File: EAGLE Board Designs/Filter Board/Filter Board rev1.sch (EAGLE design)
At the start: 118 parts, among them J4 CONNECTOR-40__, J5 CONNECTOR-40__, U10 MAX7400, U11 MAX7400, U19 MAX7400, U20 MAX7400, U21 MAX7400, U22 MAX7400, U23 MAX7400, U24 MAX7400, U6 MAX7400, U7 MAX7400, U8 MAX7400, U9 MAX7400

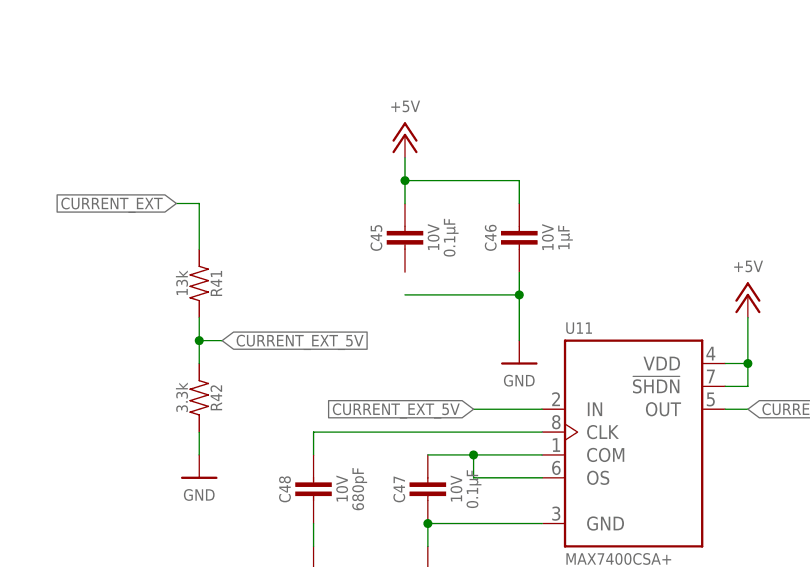
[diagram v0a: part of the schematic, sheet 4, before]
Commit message: quick fix
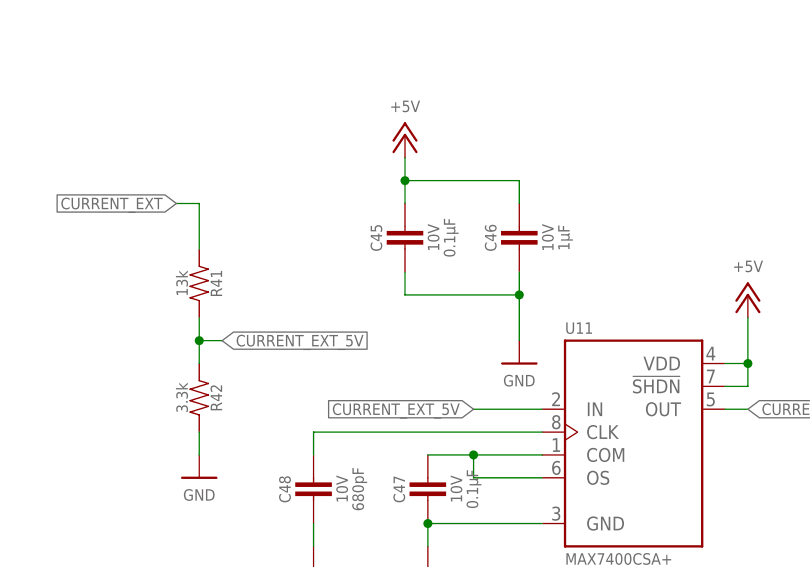
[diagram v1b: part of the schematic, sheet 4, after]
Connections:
- net GND: now also C45.2
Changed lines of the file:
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@@
 <pinref part="P139" gate="1" pin="GND"/>
 <pinref part="C46" gate="G$1" pin="2"/>
+<pinref part="C45" gate="G$1" pin="2"/>
+<wire x1="55.88" y1="53.34" x2="55.88" y2="50.8" width="0.1524" layer="91"/>
 </segment>
 <segment>

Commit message: inverted design
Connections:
- removed net GND1: R12.2, R16.2
- removed net GND2: R14.2, R18.2, R42.2, R44.2
- net GND: now also R12.2, R14.2, R16.2, R18.2, R44.2
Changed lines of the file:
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@@
 <pinref part="C10" gate="G$1" pin="2"/>
+</segment>
+<segment>
+<pinref part="P15" gate="1" pin="GND"/>
+<pinref part="R16" gate="G$1" pin="2"/>
+<wire x1="40.64" y1="73.66" x2="40.64" y2="76.2" width="0.1524" layer="91"/>
+</segment>
+<segment>
+<pinref part="P12" gate="1" pin="GND"/>
+<pinref part="R12" gate="G$1" pin="2"/>
+<wire x1="162.56" y1="124.46" x2="162.56" y2="127" width="0.1524" layer="91"/>
+</segment>
+<segment>
+<pinref part="P14" gate="1" pin="GND"/>
+<pinref part="R14" gate="G$1" pin="2"/>
+<wire x1="162.56" y1="76.2" x2="162.56" y2="78.74" width="0.1524" layer="91"/>
+</segment>
+<segment>
+<pinref part="R18" gate="G$1" pin="2"/>
+<pinref part="P16" gate="1" pin="GND"/>
+<wire x1="157.48" y1="177.8" x2="157.48" y2="175.26" width="0.1524" layer="91"/>
 </segment>
 </net>
@@
 </segment>
 </net>
-<net name="GND1" class="0">
-<segment>
-<wire x1="162.56" y1="127" x2="162.56" y2="124.46" width="0.1524" layer="91"/>
-<pinref part="P12" gate="1" pin="GND"/>
-<pinref part="R12" gate="G$1" pin="2"/>
-</segment>
-<segment>
-<wire x1="40.64" y1="76.2" x2="40.64" y2="73.66" width="0.1524" layer="91"/>
-<pinref part="P15" gate="1" pin="GND"/>
-<pinref part="R16" gate="G$1" pin="2"/>
-</segment>
-</net>
 <net name="SPN_POT_5_EXT_5V" class="0">
 <segment>
@@
 <label x="198.12" y="149.86" size="1.27" layer="95" font="vector" rot="R180" xref="yes"/>
 <pinref part="R20" gate="G$1" pin="1"/>
-</segment>
-</net>
-<net name="GND2" class="0">
-<segment>
-<wire x1="162.56" y1="78.74" x2="162.56" y2="76.2" width="0.1524" layer="91"/>
-<pinref part="P14" gate="1" pin="GND"/>
-<pinref part="R14" gate="G$1" pin="2"/>
-</segment>
-<segment>
-<wire x1="157.48" y1="177.8" x2="157.48" y2="175.26" width="0.1524" layer="91"/>
-<pinref part="P16" gate="1" pin="GND"/>
-<pinref part="R18" gate="G$1" pin="2"/>
 </segment>
 </net>
@@
 <junction x="226.06" y="162.56"/>
 </segment>
+<segment>
+<pinref part="P149" gate="1" pin="GND"/>
+<pinref part="R44" gate="G$1" pin="2"/>
+<wire x1="200.66" y1="167.64" x2="200.66" y2="172.72" width="0.1524" layer="91"/>
+</segment>
 </net>
 <net name="LOAD_RL_EXT_5V" class="0">
@@
 </segment>
 </net>
-<net name="GND2" class="0">
-<segment>
-<wire x1="33.02" y1="35.56" x2="33.02" y2="33.02" width="0.1524" layer="91"/>
-<pinref part="P148" gate="1" pin="GND"/>
-<pinref part="R42" gate="G$1" pin="2"/>
-</segment>
-<segment>
-<wire x1="200.66" y1="172.72" x2="200.66" y2="167.64" width="0.1524" layer="91"/>
-<pinref part="P149" gate="1" pin="GND"/>
-<pinref part="R44" gate="G$1" pin="2"/>
-</segment>
-</net>

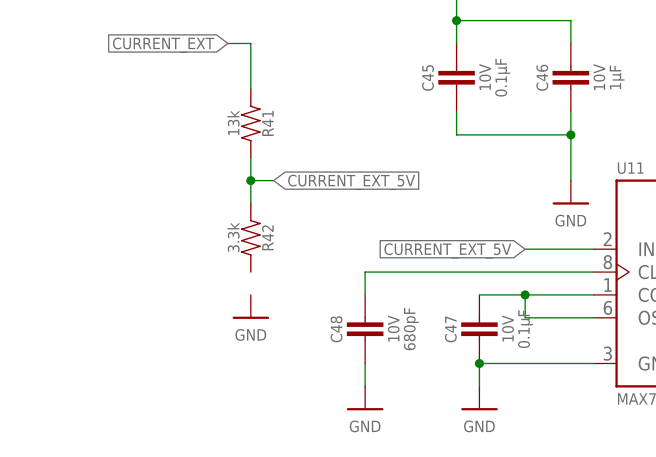
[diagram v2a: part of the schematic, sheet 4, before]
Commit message: embarassing
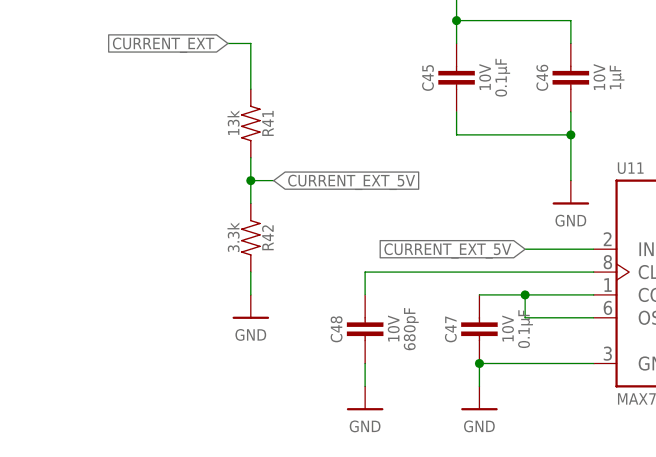
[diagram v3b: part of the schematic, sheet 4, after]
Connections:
- net GND: now also R42.2
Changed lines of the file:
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@@
 <wire x1="200.66" y1="167.64" x2="200.66" y2="172.72" width="0.1524" layer="91"/>
+</segment>
+<segment>
+<pinref part="P148" gate="1" pin="GND"/>
+<pinref part="R42" gate="G$1" pin="2"/>
+<wire x1="33.02" y1="33.02" x2="33.02" y2="35.56" width="0.1524" layer="91"/>
 </segment>
 </net>
